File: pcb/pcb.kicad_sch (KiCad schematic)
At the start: 38 parts, among them J1 Conn_01x04_Pin, J2 Conn_01x06_Pin, U1 XIAO-ESP32-C5-DIP, U10 XIAO-ESP32-C5-DIP, U11 XIAO-ESP32-C5-DIP, U12 XIAO-ESP32-C5-DIP, U13 XIAO-ESP32-C5-DIP, U14 XIAO-ESP32-C5-DIP, U15 XIAO-ESP32-C5-DIP, U17 AP2112K-3.3, U18 XIAO-ESP32-C5-DIP, U2 XIAO-ESP32-C5-DIP, U3 XIAO-ESP32-C5-DIP, U4 XIAO-ESP32-C5-DIP, U5 XIAO-ESP32-C5-DIP, U6 XIAO-ESP32-C5-DIP, U7 XIAO-ESP32-C5-DIP, U8 XIAO-ESP32-C5-DIP, U9 XIAO-ESP32-C5-DIP

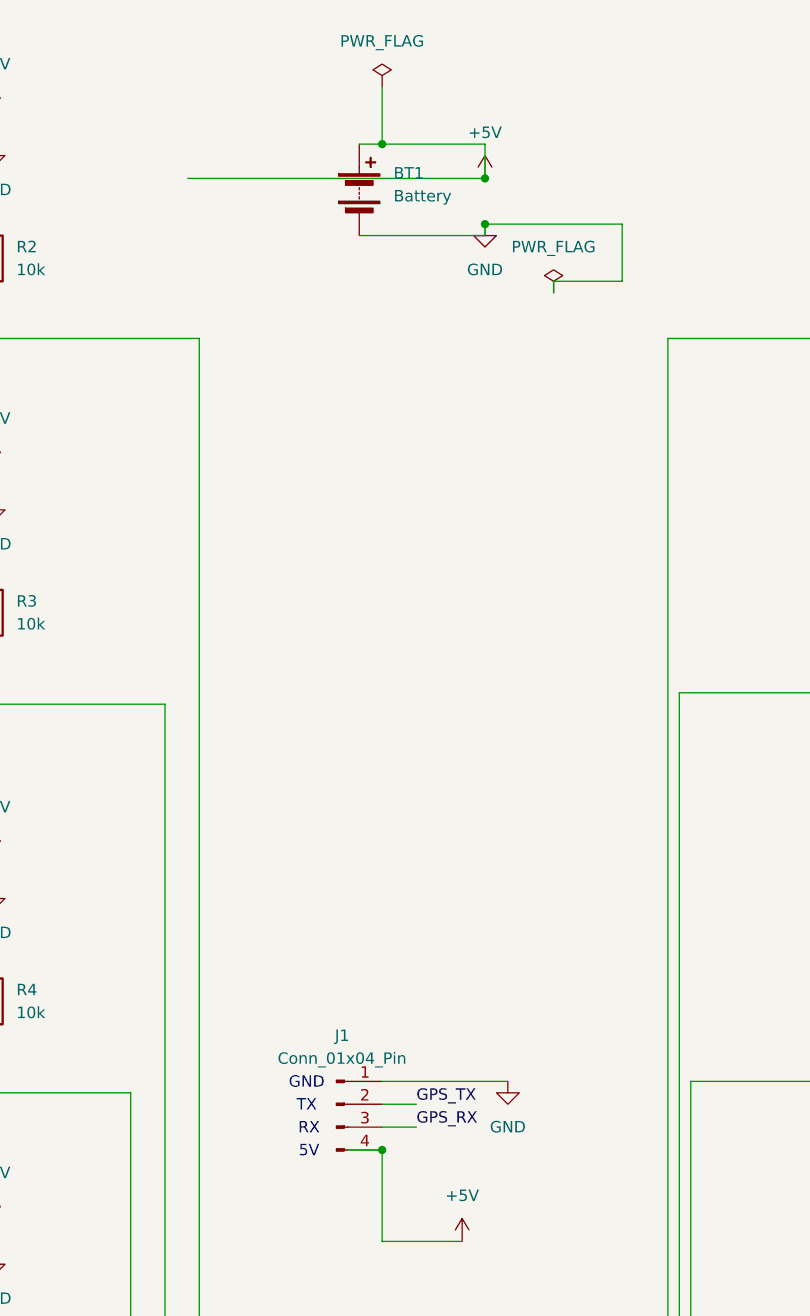
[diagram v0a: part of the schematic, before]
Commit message: tidy up warnings
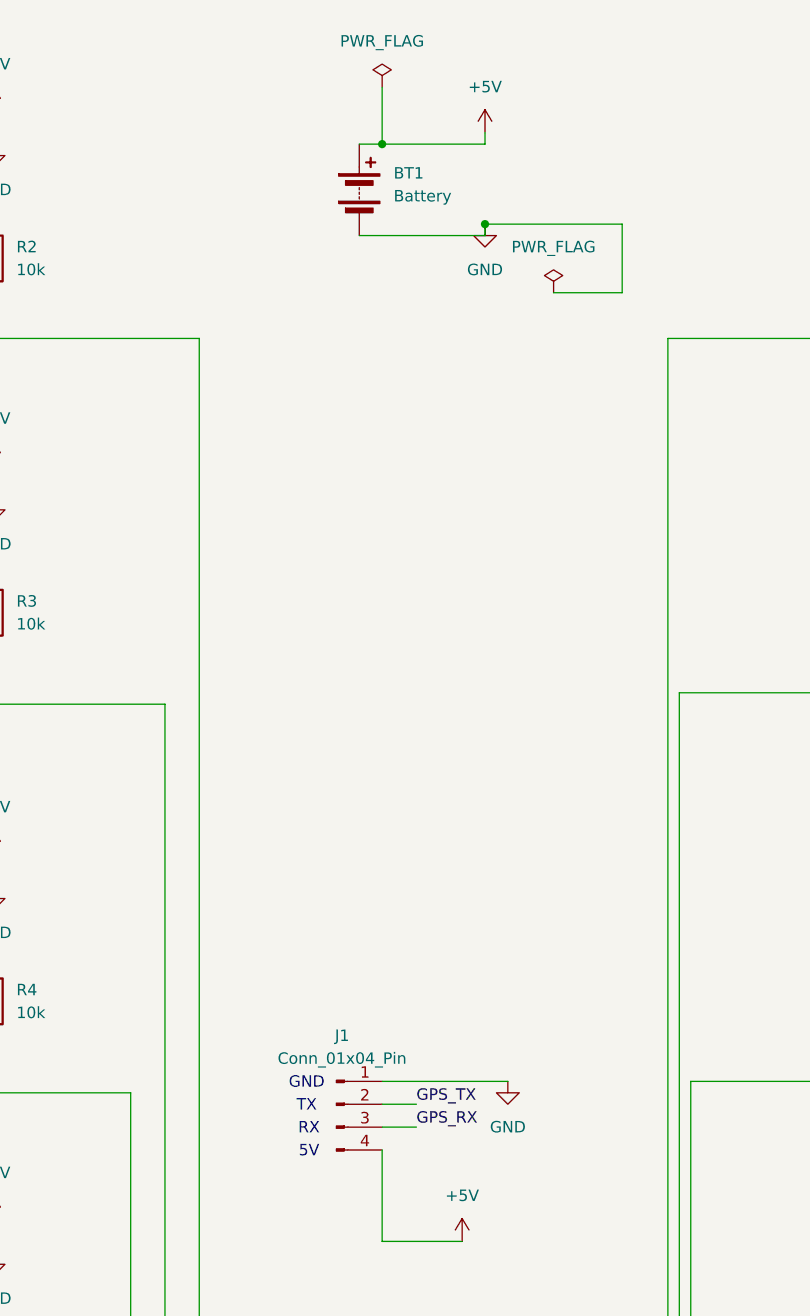
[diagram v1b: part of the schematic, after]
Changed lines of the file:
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@@
 	)
 	(junction
-		(at 130.81 138.43)
-		(diameter 0)
-		(color 0 0 0 0)
-	)
-	(junction
-		(at 142.24 30.48)
-		(diameter 0)
-		(color 0 0 0 0)
-	)
-	(junction
 		(at 87.63 252.73)
 		(diameter 0)
@@
 	(wire
 		(pts
-			(xy 127 138.43) (xy 130.81 138.43)
-		)
-		(stroke
-			(width 0)
-			(type default)
-		)
-	)
-	(wire
-		(pts
 			(xy 143.51 226.06) (xy 140.97 226.06)
 		)
@@
 	(wire
 		(pts
-			(xy 157.48 35.56) (xy 157.48 41.91)
+			(xy 157.48 35.56) (xy 157.48 43.18)
 		)
 		(stroke
@@
 	(wire
 		(pts
-			(xy 157.48 41.91) (xy 149.86 41.91)
+			(xy 157.48 43.18) (xy 149.86 43.18)
 		)
 		(stroke
@@
 	(wire
 		(pts
-			(xy 142.24 30.48) (xy 109.22 30.48)
-		)
-		(stroke
-			(width 0)
-			(type default)
-		)
-	)
-	(wire
-		(pts
 			(xy 153.67 248.92) (xy 162.56 248.92)
 		)
@@
 	(wire
 		(pts
-			(xy 149.86 41.91) (xy 149.86 43.18)
-		)
-		(stroke
-			(width 0)
-			(type default)
-		)
-	)
-	(wire
-		(pts
 			(xy 99.06 321.31) (xy 119.38 321.31)
 		)
@@
 	(wire
 		(pts
-			(xy 142.24 26.67) (xy 142.24 30.48)
+			(xy 142.24 26.67) (xy 142.24 25.4)
 		)
 		(stroke
@@
 	(symbol
 		(lib_id "power:+5V")
-		(at 142.24 30.48 0)
+		(at 142.24 25.4 0)
 		(unit 1)
 		(body_style 1)
@@
 		(fields_autoplaced yes)
 		(property "Reference" "#PWR01"
-			(at 142.24 34.29 0)
+			(at 142.24 29.21 0)
 			(hide yes)
 			(show_name no)
@@
 		)
 		(property "Value" "+5V"
-			(at 142.24 25.4 0)
+			(at 142.24 20.32 0)
 			(show_name no)
 			(do_not_autoplace no)
@@
 		)
 		(property "Footprint" ""
-			(at 142.24 30.48 0)
+			(at 142.24 25.4 0)
 			(hide yes)
 			(show_name no)
@@
 		)
 		(property "Datasheet" ""
-			(at 142.24 30.48 0)
+			(at 142.24 25.4 0)
 			(hide yes)
 			(show_name no)
@@
 		)
 		(property "Description" "Power symbol creates a global label with name \"+5V\""
-			(at 142.24 30.48 0)
+			(at 142.24 25.4 0)
 			(hide yes)
 			(show_name no)

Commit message: more progress with the PCB layout
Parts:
- BT1: footprint Connector_PinHeader_2.54mm:PinHeader_1x02_P2.54mm_Horizontal -> Connector_PinHeader_2.54mm:PinHeader_1x02_P2.54mm_Vertical
- J1: footprint Connector_PinHeader_2.54mm:PinHeader_1x04_P2.54mm_Horizontal -> Connector_PinHeader_2.54mm:PinHeader_1x04_P2.54mm_Vertical
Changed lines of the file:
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@@
 			)
 		)
-		(property "Footprint" "Connector_PinHeader_2.54mm:PinHeader_1x04_P2.54mm_Horizontal"
+		(property "Footprint" "Connector_PinHeader_2.54mm:PinHeader_1x04_P2.54mm_Vertical"
 			(at 125.73 133.35 0)
 			(hide yes)
@@
 			)
 		)
-		(property "Footprint" "Connector_PinHeader_2.54mm:PinHeader_1x02_P2.54mm_Horizontal"
+		(property "Footprint" "Connector_PinHeader_2.54mm:PinHeader_1x02_P2.54mm_Vertical"
 			(at 128.27 30.226 90)
 			(hide yes)
